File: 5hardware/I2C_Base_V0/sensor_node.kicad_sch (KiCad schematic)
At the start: 66 parts, among them J2 PJ-320D-A, J3 Conn_02x06_Top_Bottom, J4 Conn_01x19_Socket, J5 Conn_01x19_Socket, J6 Conn_01x06_Socket, J7 Conn_01x04_Pin, J8 Conn_01x04_Pin, P1 S3B-PH-SM4-TB, P2 S4B-PH-SM4-TB, P3 S3B-PH-SM4-TB, Q2 Si2371EDS, Q3 Si2371EDS, SW2 SW_Push, SW3 SW_Push, U10 ESP-12F, U12 APDS-9960, U14 DS3231M, U3 CR2450, U4 CH32V003F4P6, U5 SHT31-DIS, U6 DS1307Z+, U7 XC6206PxxxMR, U8 TPL5110, U9 BH1750FVI-TR, Y1 Crystal, Y2 Crystal

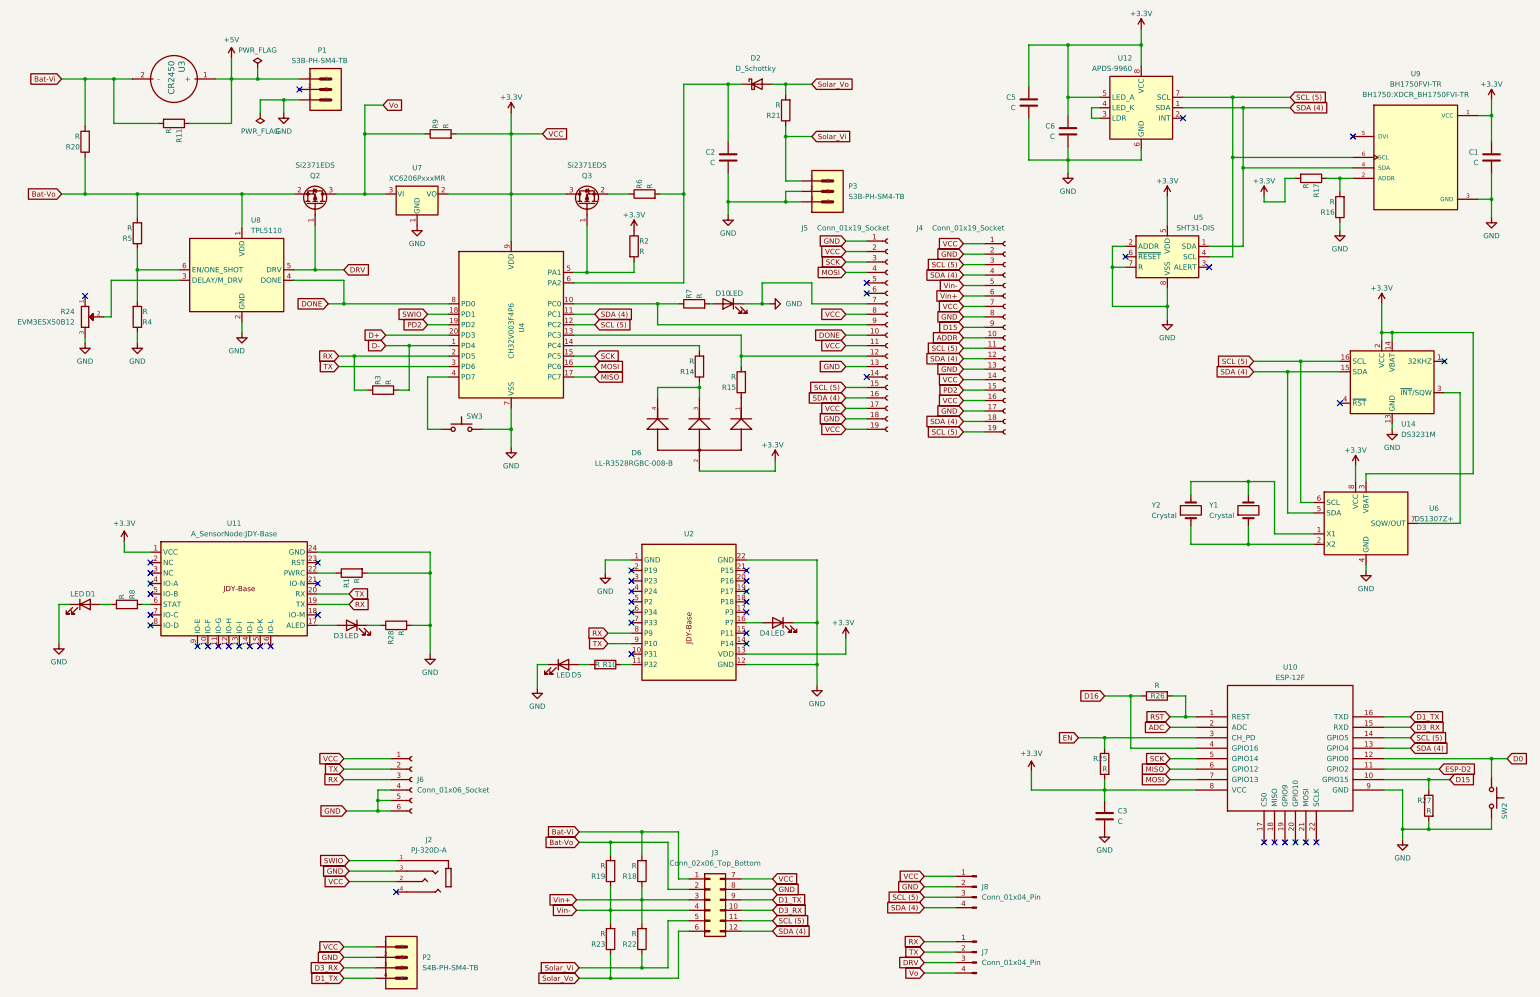
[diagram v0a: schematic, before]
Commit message: update PCB.
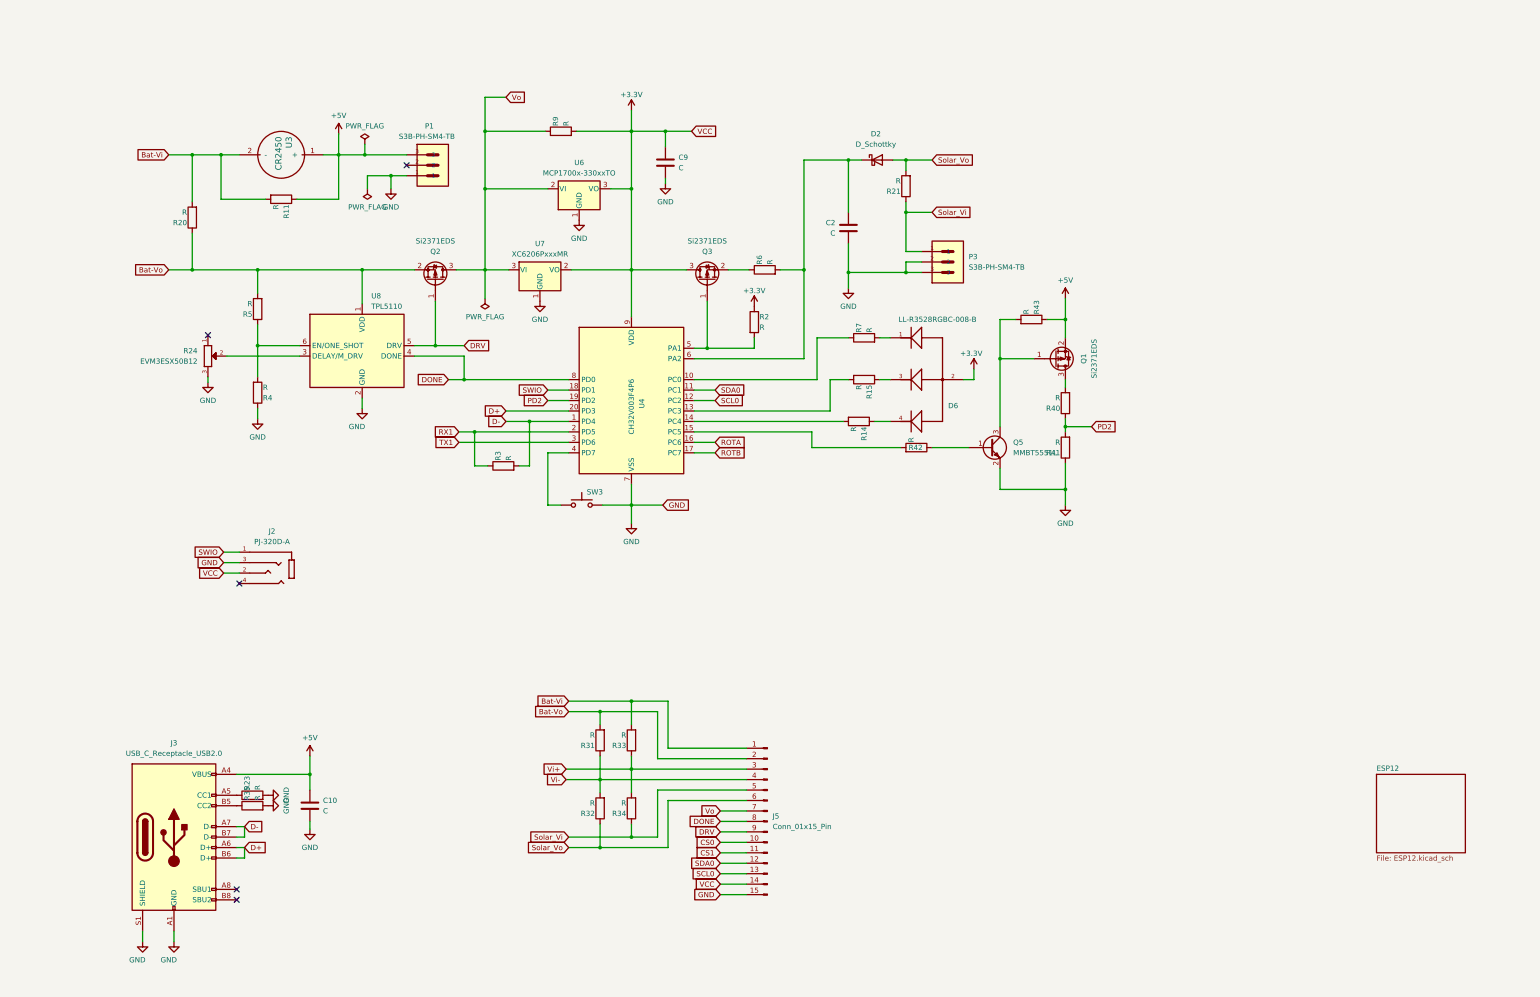
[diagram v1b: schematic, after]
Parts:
- removed C1, C3, C5, C6: C, Capacitor_SMD:C_1206_3216Metric, symbol Device:C
- removed D1, D10, D3, D4, D5: LED, LED_SMD:LED_0603_1608Metric, symbol Device:LED
- removed J3: Conn_02x06_Top_Bottom, Connector_PinHeader_2.54mm:PinHeader_2x06_P2.54mm_Vertical, symbol Connector_Generic:Conn_02x06_Top_Bottom
- removed J4, J5: Conn_01x19_Socket, Connector_PinSocket_2.54mm:PinSocket_1x19_P2.54mm_Vertical, symbol Connector:Conn_01x19_Socket
- removed J6: Conn_01x06_Socket, Connector_PinHeader_2.00mm:PinHeader_1x06_P2.00mm_Vertical, symbol Connector:Conn_01x06_Socket
- removed J7, J8: Conn_01x04_Pin, Connector_PinHeader_1.27mm:PinHeader_1x04_P1.27mm_Vertical, symbol Connector:Conn_01x04_Pin
- removed P2: S4B-PH-SM4-TB, S4B-PH:JST_S4B-PH-SM4-TB, symbol JST_S4B-PH:S4B-PH-SM4-TB
- removed R1, R16, R17, R18, R19, R22: R, Resistor_SMD:R_0603_1608Metric, symbol Device:R
- removed R10, R28, R8: R, Resistor_SMD:R_0805_2012Metric, symbol Device:R
- removed R25, R26, R27: R, Resistor_SMD:R_1206_3216Metric, symbol Device:R
- removed SW2: SW_Push, Button_Switch_SMD:SW_SPST_PTS810, symbol Switch:SW_Push
- removed U10: ESP-12F, A_SensorNode:ESP12_SMD, symbol ESP8266:ESP-12F
- removed U11: ~, A_SensorNode:JDY-Base, symbol A_SensorNode:JDY-Base
- removed U12: APDS-9960, Sensor:Avago_APDS-9960, symbol Sensor:APDS-9960
- removed U14: DS3231M, Package_SO:SOIC-16W_7.5x10.3mm_P1.27mm, symbol Timer_RTC:DS3231M
- removed U2: ~, A_SensorNode:E104-BT07, symbol A_SensorNode:E104-BT07
- removed U5: SHT31-DIS, Sensor_Humidity:Sensirion_DFN-8-1EP_2.5x2.5mm_P0.5mm_EP1.1x1.7mm, symbol Sensor_Humidity:SHT31-DIS
- removed U6: DS1307Z+, Package_SO:SOIC-8_3.9x4.9mm_P1.27mm, symbol Timer_RTC:DS1307Z+
- removed U9: BH1750FVI-TR, BH1750:XDCR_BH1750FVI-TR, symbol BH1750FVI-TR:BH1750FVI-TR
- removed Y1: Crystal, Crystal:Crystal_SMD_3215-2Pin_3.2x1.5mm, symbol Device:Crystal
- removed Y2: Crystal, Crystal:Crystal_Round_D1.5mm_Vertical, symbol Device:Crystal
- added C10, C9: C, Capacitor_SMD:C_0805_2012Metric, symbol Device:C
- added J3: USB_C_Receptacle_USB2.0, Connector_USB:USB_C_Receptacle_G-Switch_GT-USB-7010ASV, symbol Connector:USB_C_Receptacle_USB2.0
- added J5: Conn_01x15_Pin, Connector_PinHeader_2.54mm:PinHeader_1x15_P2.54mm_Vertical, symbol Connector:Conn_01x15_Pin
- added Q1: Si2371EDS, Package_TO_SOT_SMD:SOT-23, symbol Transistor_FET:Si2371EDS
- added Q5: MMBT5551L, Package_TO_SOT_SMD:SOT-23, symbol Transistor_BJT:MMBT5551L
- added R31, R32, R33, R34: R, Resistor_SMD:R_0603_1608Metric, symbol Device:R
- added R35, R40, R41, R42, R43: R, Resistor_SMD:R_0805_2012Metric, symbol Device:R
- added U6: MCP1700x-330xxTO, Package_TO_SOT_THT:TO-92_Inline, symbol Regulator_Linear:MCP1700x-330xxTO
- C2: footprint Capacitor_SMD:C_1206_3216Metric -> Capacitor_SMD:C_0805_2012Metric
- R14, R15, R2, R3: footprint Resistor_SMD:R_1206_3216Metric -> Resistor_SMD:R_0805_2012Metric
- R23: footprint Resistor_SMD:R_0603_1608Metric -> Resistor_SMD:R_0805_2012Metric
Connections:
- net Vin- is gone; now on net GND: R23.2
- net +3.3V: now also C9.1, J5.14 (Pin_14), U6.3 (VO)
- net +5V: now also C10.1, J3.A4 (VBUS), J3.A9 (VBUS), J3.B4 (VBUS), J3.B9 (VBUS), Q1.2 (S), R43.1
- net Bat-Vi: now also J5.1 (Pin_1), R33.2
- net Bat-Vo: now also J5.2 (Pin_2), R31.2
- net D+: now also J3.A6 (D+), J3.B6 (D+)
- net D-: now also J3.A7 (D-), J3.B7 (D-)
- net DONE: now also J5.8 (Pin_8)
- net DRV: now also J5.9 (Pin_9)
- net GND: now also C10.2, C9.2, J3.A1 (GND), J3.A12 (GND), J3.B1 (GND), J3.B12 (GND), J3.S1 (SHIELD), J5.15 (Pin_15), Q5.2 (E), R35.2, R41.1, U6.1 (GND)
- net PD2: now also R40.1, R41.2
- net Solar_Vi: now also J5.5 (Pin_5), R34.1
- net Solar_Vo: now also J5.6 (Pin_6), R32.1; no longer R23.1
- net Vo: now also J5.7 (Pin_7), U6.2 (VI)
- net at R15.1: now also D6.3; no longer D6.1
- net at R7.2: now also D6.1
- net at D6.4, R14.1: no longer D6.3
- net MISO renamed ROTB
- net MOSI renamed ROTA
- net RX renamed RX1
- net SCK: no longer names the net of U4.15 (PC5)
- net SCK: now also R42.2
- net SCL (5) renamed SCL0
- net SCL0: now also J5.13 (Pin_13)
- net SDA (4) renamed SDA0
- net SDA0: now also J5.12 (Pin_12)
- net TX renamed TX1
- new net: J3.B5 (CC2), R35.1
- new net: Q1.1 (G), Q5.3 (C), R43.2
- new net: Q1.3 (D), R40.2
- new net: Q5.1 (B), R42.1
- new net: J3.A5 (CC1), R23.1
- new net CS0: J5.10 (Pin_10)
- new net CS1: J5.11 (Pin_11)
- new net Vi+: J5.3 (Pin_3), R33.1, R34.2
- new net Vi-: J5.4 (Pin_4), R31.1, R32.2
- no-connect marks 49 -> 5
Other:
- added sheet ESP12 (ESP12.kicad_sch)
- moved on the sheet: C2, D2, D6, J2, P1, P3, Q2, Q3, R11, R15, R2, R20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
